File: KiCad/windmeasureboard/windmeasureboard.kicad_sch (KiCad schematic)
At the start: 20 parts, among them J1 ESQ-120-XX-X-D-XX, U1 ESP32-S2-DEVKITC-1, U2 LM1084ISX-5.0_NOPB

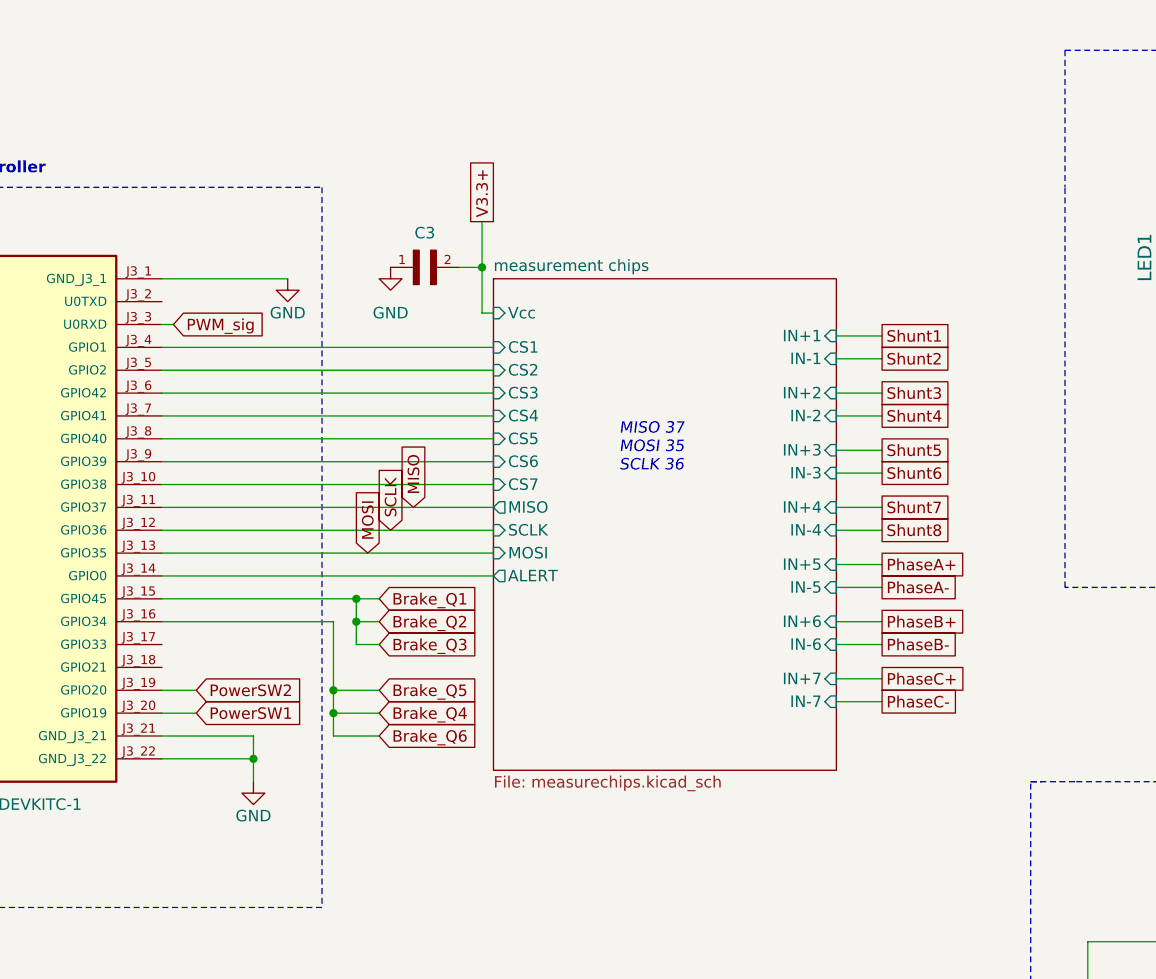
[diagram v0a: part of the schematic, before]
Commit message: WMB 2.2 pushed and ordered
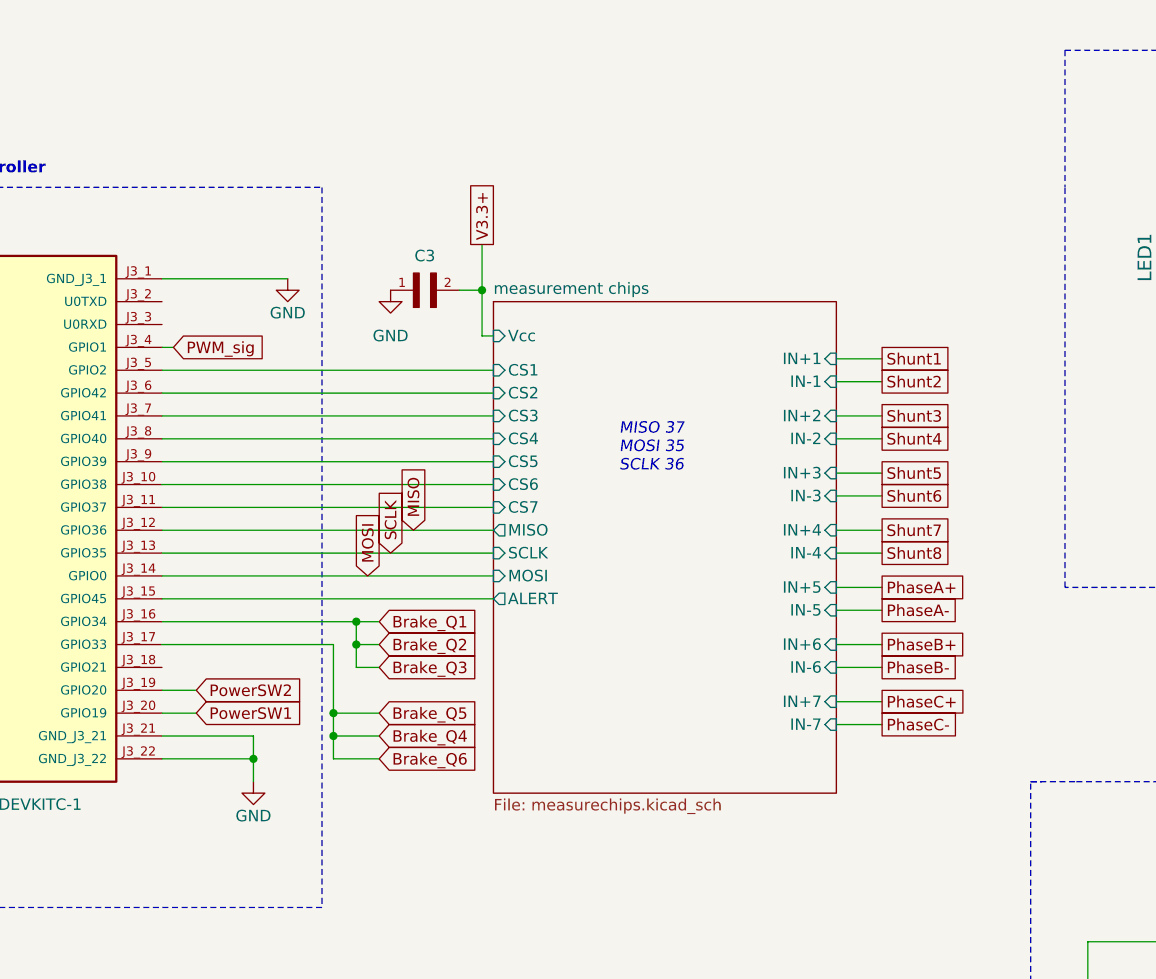
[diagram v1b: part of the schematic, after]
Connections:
- net Brake_Q1: now also U1.J3_16 (GPIO34); no longer U1.J3_15 (GPIO45)
- net Brake_Q4: now also U1.J3_17 (GPIO33); no longer U1.J3_16 (GPIO34)
- net MISO: now also U1.J3_12 (GPIO36); no longer U1.J3_11 (GPIO37)
- net MOSI: now also U1.J3_14 (GPIO0); no longer U1.J3_13 (GPIO35)
- net PWM_sig: now also U1.J3_4 (GPIO1); no longer U1.J3_3 (U0RXD)
- net SCLK: now also U1.J3_13 (GPIO35); no longer U1.J3_12 (GPIO36)
- net measurement chips/ALERT: now also U1.J3_15 (GPIO45); no longer U1.J3_14 (GPIO0)
- net measurement chips/CS1: now also U1.J3_5 (GPIO2); no longer U1.J3_4 (GPIO1)
- net measurement chips/CS2: now also U1.J3_6 (GPIO42); no longer U1.J3_5 (GPIO2)
- net measurement chips/CS3: now also U1.J3_7 (GPIO41); no longer U1.J3_6 (GPIO42)
- net measurement chips/CS4: now also U1.J3_8 (GPIO40); no longer U1.J3_7 (GPIO41)
- net measurement chips/CS5: now also U1.J3_9 (GPIO39); no longer U1.J3_8 (GPIO40)
- net measurement chips/CS6: now also U1.J3_10 (GPIO38); no longer U1.J3_9 (GPIO39)
- net measurement chips/CS7: now also U1.J3_11 (GPIO37); no longer U1.J3_10 (GPIO38)
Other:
- moved on the sheet: C3
